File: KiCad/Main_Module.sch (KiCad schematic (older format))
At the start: 44 parts, among them IC1 ATMEGA88-A, Q1 Q_NMOS_GDS, Q2 Q_NMOS_GDS, Q3 Q_NMOS_GDS, Q4 Q_NMOS_GDS, U1 LM324, U2 7805

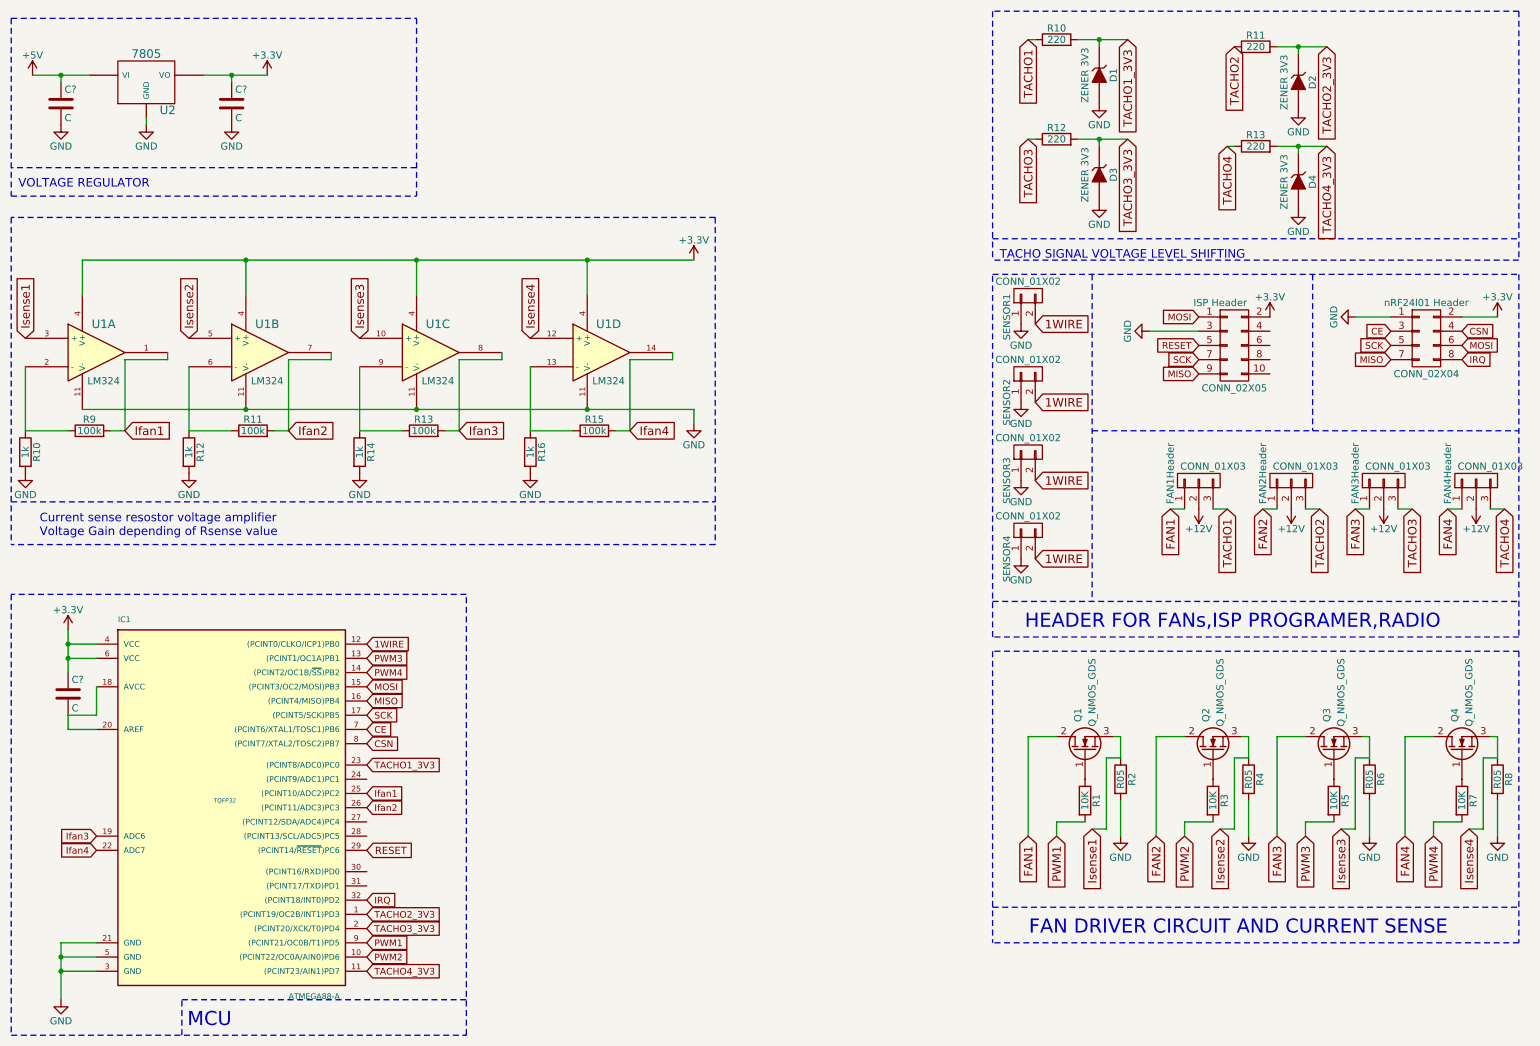
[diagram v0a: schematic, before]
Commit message: some changes on mainmodule
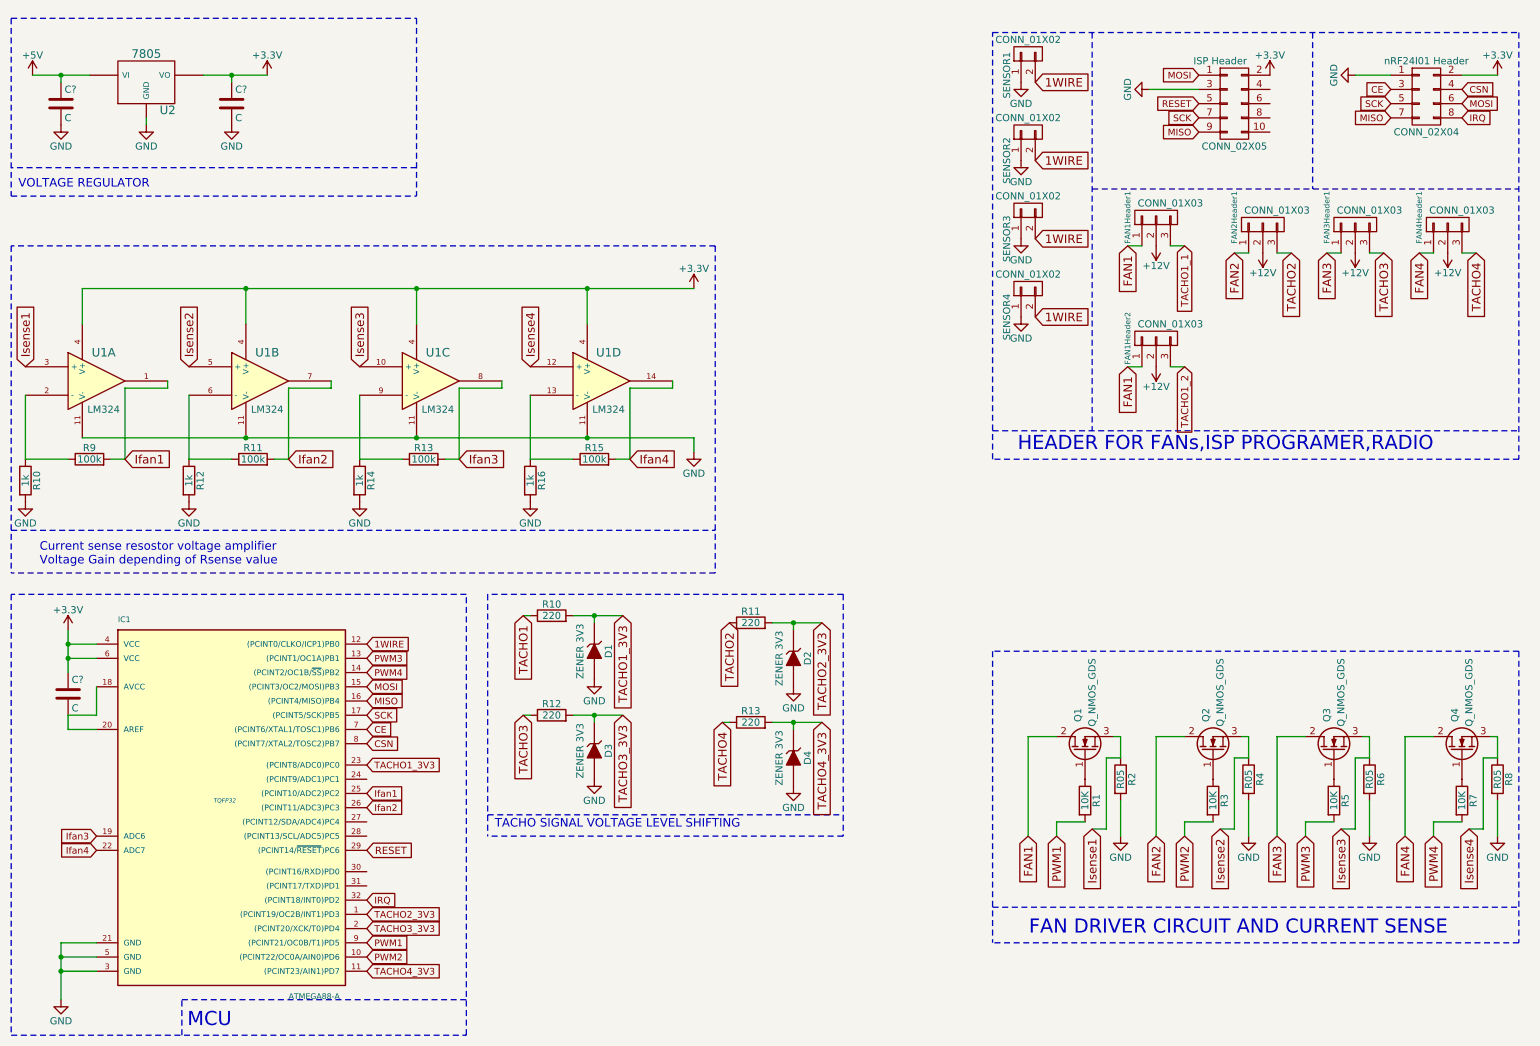
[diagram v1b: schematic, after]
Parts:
- added FAN1Header2: CONN_01X03, symbol CONN_01X03
- renumbered FAN1Header to FAN1Header1, FAN2Header to FAN2Header1, FAN3Header to FAN3Header1, FAN4Header to FAN4Header1
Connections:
- net +12V: now also FAN1Header2.2 (P2)
- net FAN1: now also FAN1Header2.1 (P1)
- net TACHO1: no longer FAN1Header1.3 (P3)
- new net TACHO1_1: FAN1Header1.3 (P3)
- new net TACHO1_2: FAN1Header2.3 (P3)
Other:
- moved on the sheet: D1, D2, D3, D4, FAN1Header1, FAN2Header1, FAN3Header1, FAN4Header1, ISP Header, R10, R11, R12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
